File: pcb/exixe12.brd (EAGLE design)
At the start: 20 x 40 mm, 42 parts

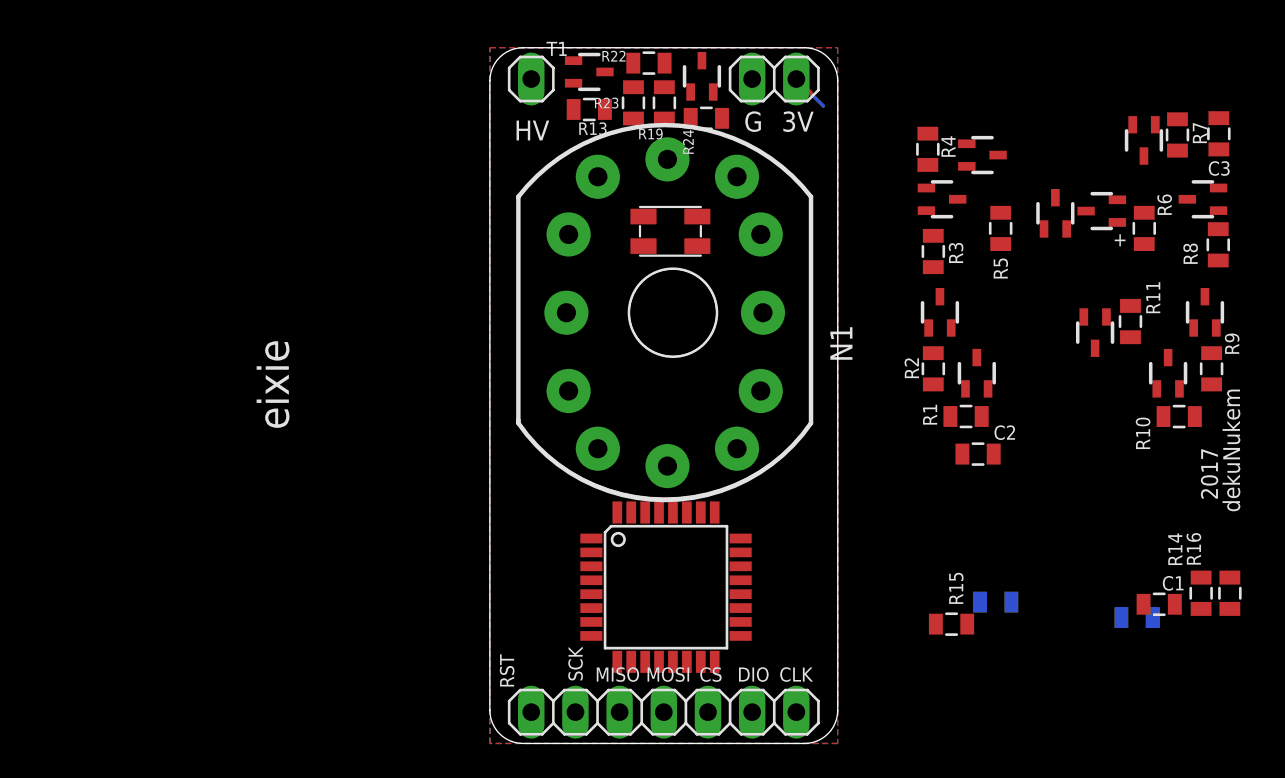
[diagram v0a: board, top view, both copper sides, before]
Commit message: sending out
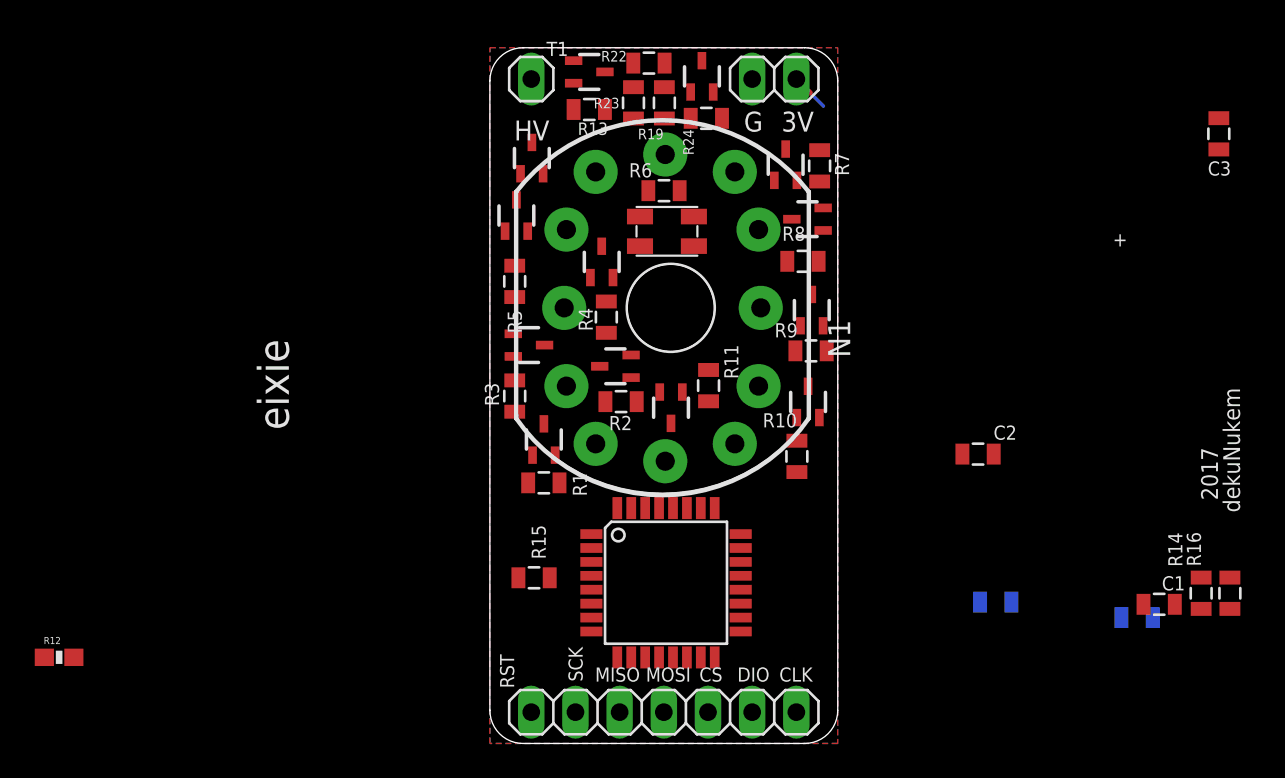
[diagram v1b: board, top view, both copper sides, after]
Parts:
- added R12: (no value), SparkFun-Resistors:0603-RES
- moved Q6 32.9 mm to (2.41, 33.7), turned to 0 degrees
- moved Q5 31.0 mm to (1.52, 30.4)
- moved R5 28.1 mm to (1.43, 26.6)
- moved R6 27.7 mm to (10.0, 31.8), turned to 180 degrees
- moved R3 25.5 mm to (1.43, 20.0), turned to 270 degrees
- moved Q3 25.2 mm to (2.25, 22.9)
- moved Q1 25.2 mm to (3.10, 17.5)
- moved Q11 24.8 mm to (10.4, 19.3)
- moved R1 24.6 mm to (3.10, 15.0), turned to 180 degrees
- moved R11 24.5 mm to (12.6, 20.6)
- moved R15 24.2 mm to (2.54, 9.53)
- moved R8 23.9 mm to (18.0, 27.7), turned to 0 degrees
- moved R9 23.1 mm to (18.5, 22.6), turned to 180 degrees
- moved Q8 22.8 mm to (18.3, 30.1)
- moved Q4 22.7 mm to (6.43, 27.7), turned to 0 degrees
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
